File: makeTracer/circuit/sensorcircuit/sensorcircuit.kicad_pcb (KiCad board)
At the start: 2 copper layers, 90 x 80.1 mm, 38 parts, among them J1 Maincircuit, U1 LBR-127HLD, U2 RPR-220, U3 4052, U4 RPR-220, U5 LBR-127HLD, U6 LBR-127HLD, U7 LBR-127HLD, U8 LBR-127HLD, U9 LBR-127HLD

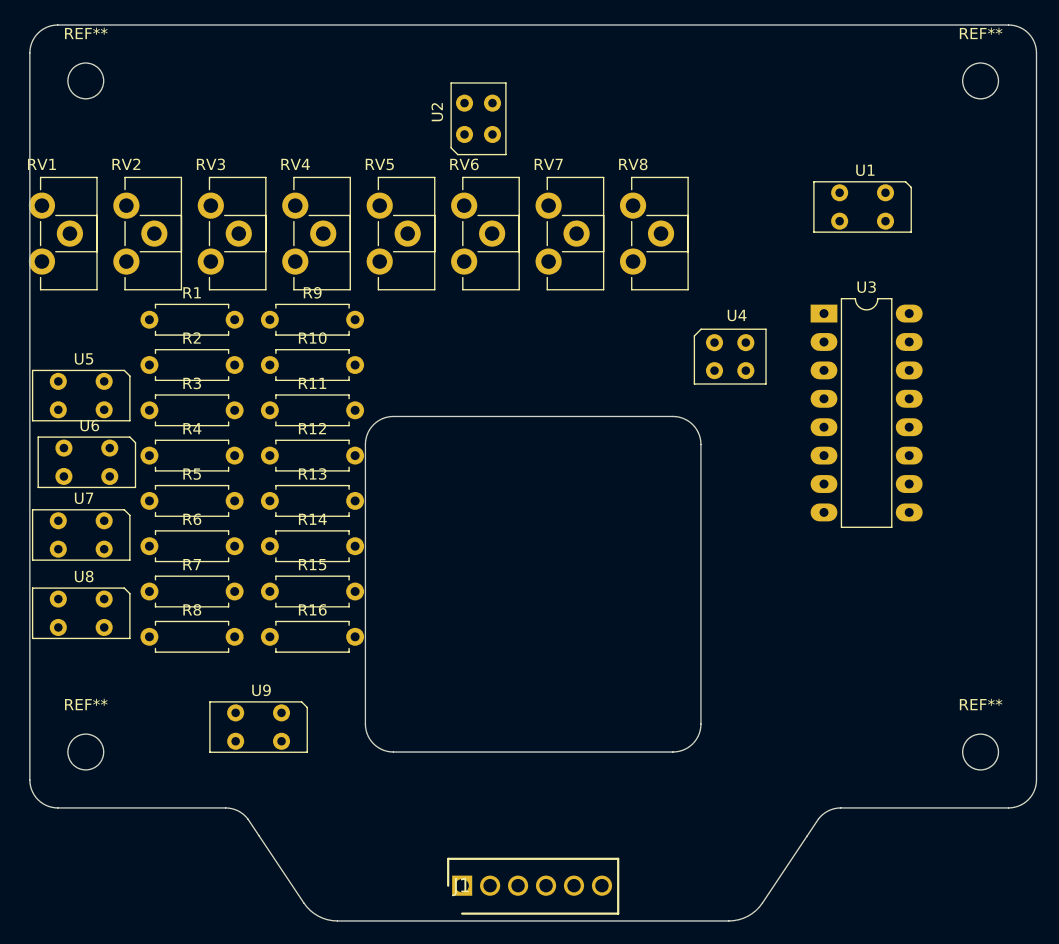
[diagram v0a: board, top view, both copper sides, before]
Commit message: complete: circuit
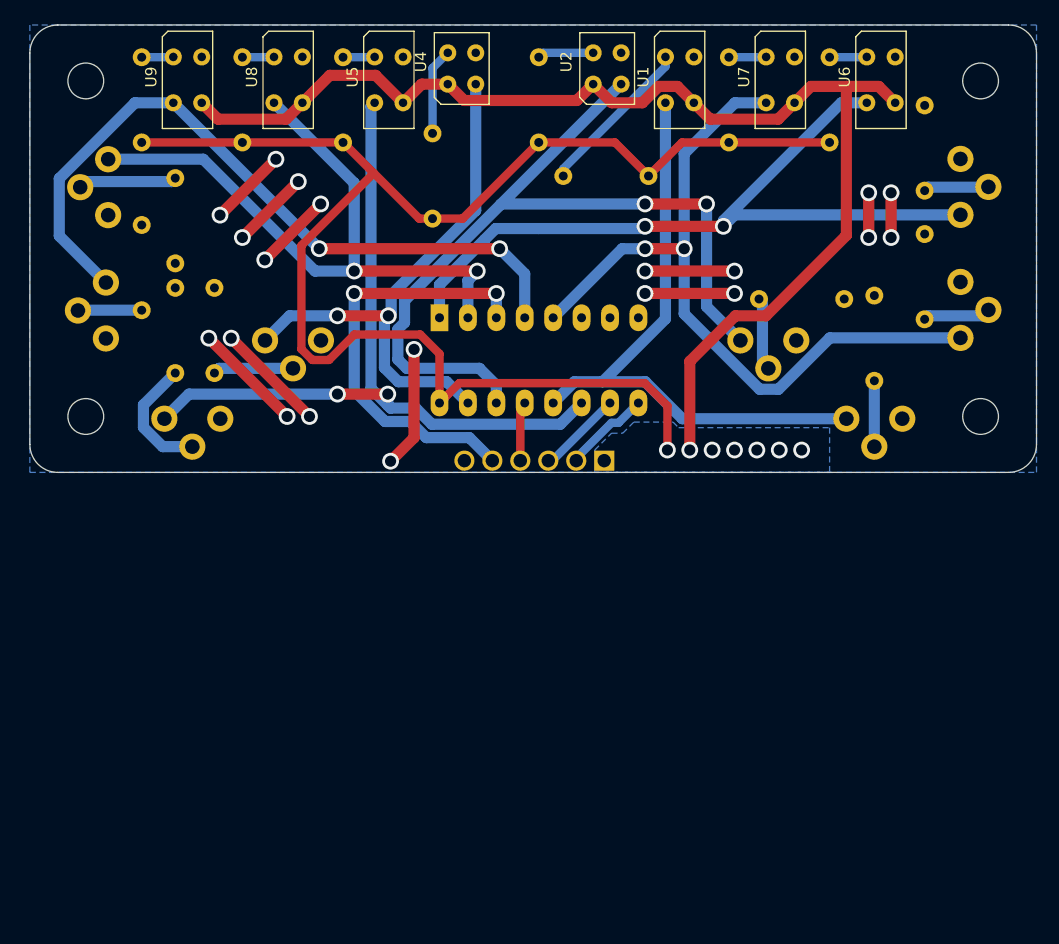
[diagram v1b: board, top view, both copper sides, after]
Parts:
- J1, R1, R10, R11, R12, R13, R14, R15, R16, R2, R3, R4, R5, R6, R7, R8, R9, RV1, RV2, RV3, RV4, RV5, RV6, RV7, RV8, U3: moved to B.Cu
- moved U6 78.1 mm to (93.8, 29.3), turned to 90 degrees
- moved RV1 74.4 mm to (93.0, 55.2), turned to -90 degrees
- moved U7 73.0 mm to (84.8, 29.3), turned to 90 degrees
- moved R2 64.8 mm to (95.5, 51.8), turned to 90 degrees
- moved R10 60.6 mm to (100.0, 34.8), turned to 90 degrees
- moved R12 59.8 mm to (100.0, 46.3), turned to 90 degrees
- moved R4 56.3 mm to (85.2, 44.5)
- moved RV2 56.2 mm to (83.5, 48.2), turned to -90 degrees
- moved R9 52.5 mm to (91.5, 30.5), turned to 90 degrees
- moved RV5 51.9 mm to (103.2, 37.0)
- moved U9 51.4 mm to (31.8, 29.3), turned to 90 degrees
- moved RV8 47.6 mm to (26.8, 43.0), turned to 180 degrees
- moved R11 47.5 mm to (82.5, 30.5), turned to 90 degrees
- moved R1 46.4 mm to (75.3, 33.5), turned to 180 degrees
- moved U8 46.0 mm to (40.8, 29.3), turned to 90 degrees
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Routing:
- net VDD: track 0.00 -> 244.1 mm, vias 0 -> 7
- net /Ann_1: track 0.00 -> 76.1 mm, vias 0 -> 2
- net GND: track 0.00 -> 75.9 mm, vias 0 -> 20
- net /Dig_0: track 0.00 -> 69.8 mm, vias 0 -> 2
- net /Ann_3: track 0.00 -> 68.9 mm, vias 0 -> 2
- net /Dig_1: track 0.00 -> 67.2 mm, vias 0 -> 2
- net /Dig_3: track 0.00 -> 65.7 mm, vias 0 -> 2
- net /Dig_2: track 0.00 -> 59.7 mm, vias 0 -> 2
- net /Ann_0: track 0.00 -> 55.6 mm
- net /Ann_2: track 0.00 -> 49.4 mm, vias 0 -> 2
- net Digital_Process: track 0.00 -> 38.5 mm, vias 0 -> 2
- net Net-(R1-Pad2): track 0.00 -> 14.4 mm
- net Net-(R8-Pad1): track 0.00 -> 11.1 mm
- net Net-(R14-Pad1): track 0.00 -> 8.84 mm
- net Port_SEL2: track 0.00 -> 7.83 mm
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- added copper zone on B.Cu, net GND
- added copper zone on B.Cu, net VDD
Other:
- board size 90 x 80.1 mm -> 90 x 40 mm
- board text added: "FRONTSIDE"
- board text added: "LINE WIDTH"
